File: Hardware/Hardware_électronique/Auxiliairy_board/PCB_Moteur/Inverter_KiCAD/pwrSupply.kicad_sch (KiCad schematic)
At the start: 11 parts, among them J4 Conn_01x02_Pin, U503 AZ1117-3.3

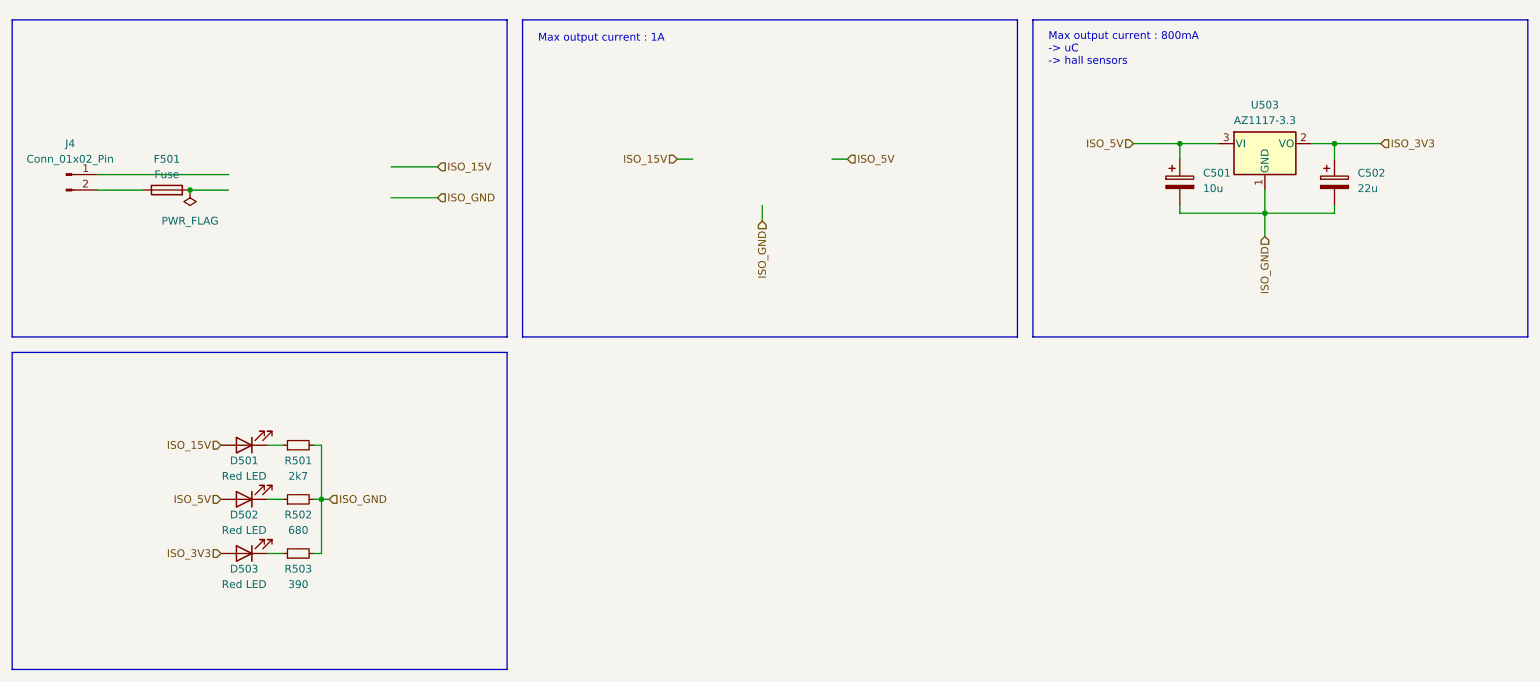
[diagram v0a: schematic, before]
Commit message: Add files via upload
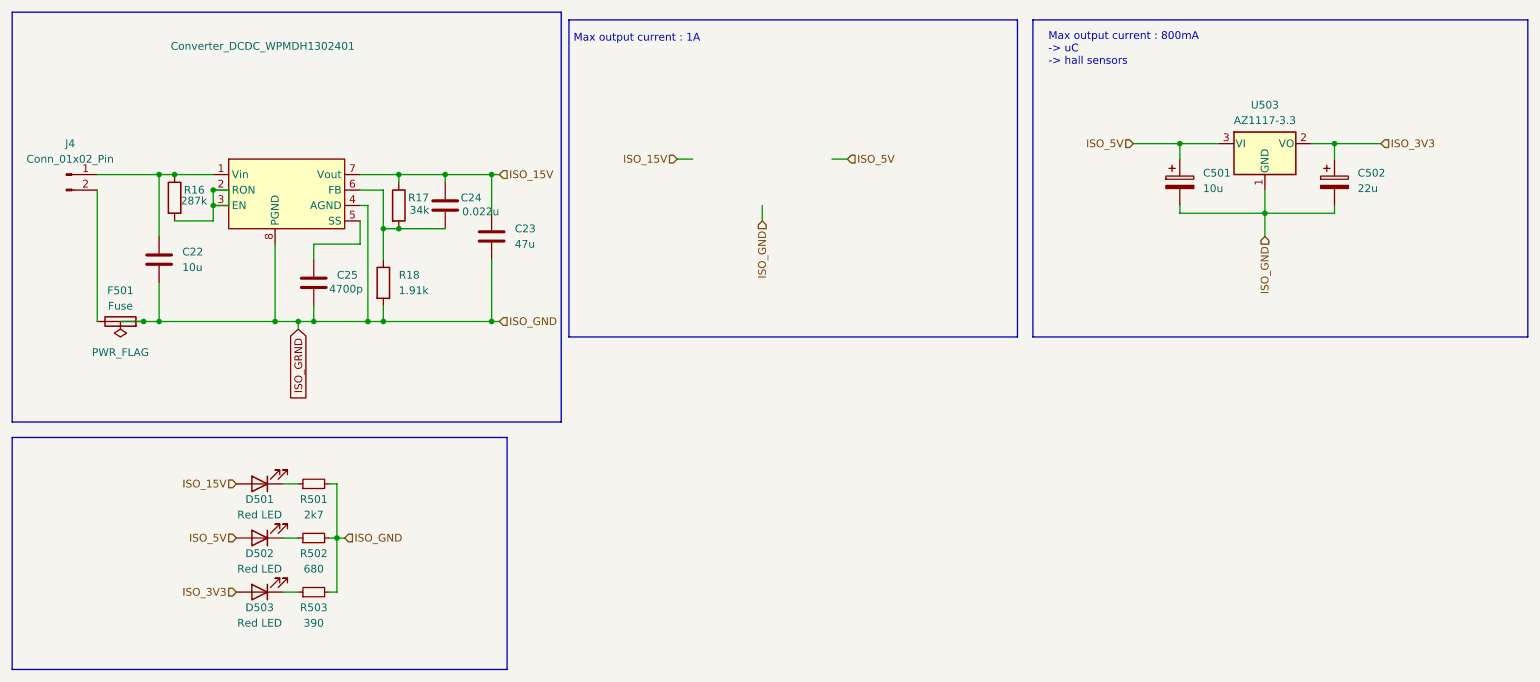
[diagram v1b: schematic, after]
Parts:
- added C22: 10u, symbol Device:C
- added C23: 47u, symbol Device:C
- added C24: 0.022u, symbol Device:C
- added C25: 4700p, symbol Device:C
- added Converter_DCDC_WPMDH1302401: ~, Custom:Converter_DCDC, symbol Custom:Converter_DCDC
- added R16: 287k, symbol Device:R
- added R17: 34k, symbol Device:R
- added R18: 1.91k, symbol Device:R
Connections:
- net ISO_GND is gone; now on net ISO_GRND: C501.2, C502.2, R501.2, R502.2, R503.2, U503.1 (GND)
- net ISO_15V: now also C23.1, C24.1, Converter_DCDC_WPMDH1302401.7 (Vout), R17.1
- net at J4.1 (Pin_1): now also C22.1, Converter_DCDC_WPMDH1302401.1 (Vin), R16.1
- net ISO_GRND: now reaches F501.2
- net ISO_GRND: now also C22.2, C23.2, C25.2, Converter_DCDC_WPMDH1302401.4 (AGND), Converter_DCDC_WPMDH1302401.8 (PGND), R18.2
- new net: Converter_DCDC_WPMDH1302401.2 (RON), Converter_DCDC_WPMDH1302401.3 (EN), R16.2
- new net: C25.1, Converter_DCDC_WPMDH1302401.5 (SS)
- new net: C24.2, Converter_DCDC_WPMDH1302401.6 (FB), R17.2, R18.1
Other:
- moved on the sheet: D501, D502, D503, F501, R501, R502, R503
